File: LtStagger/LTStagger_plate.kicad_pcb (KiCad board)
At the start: 2 copper layers, 155 x 112 mm, 26 parts, among them K0 K00, K1 K01, K10 K10, K11 K11, K12 K12, K2 K02, K20 K20, K21 K21, K22 K22, K30 K30, K31 K31, K32 K32, K33 K33, K40 K40, K41 K41, K42 K42, K43 K43, K50 K50, K51 K51, K53 K53, SW1 Rotary_Encoder_Switch

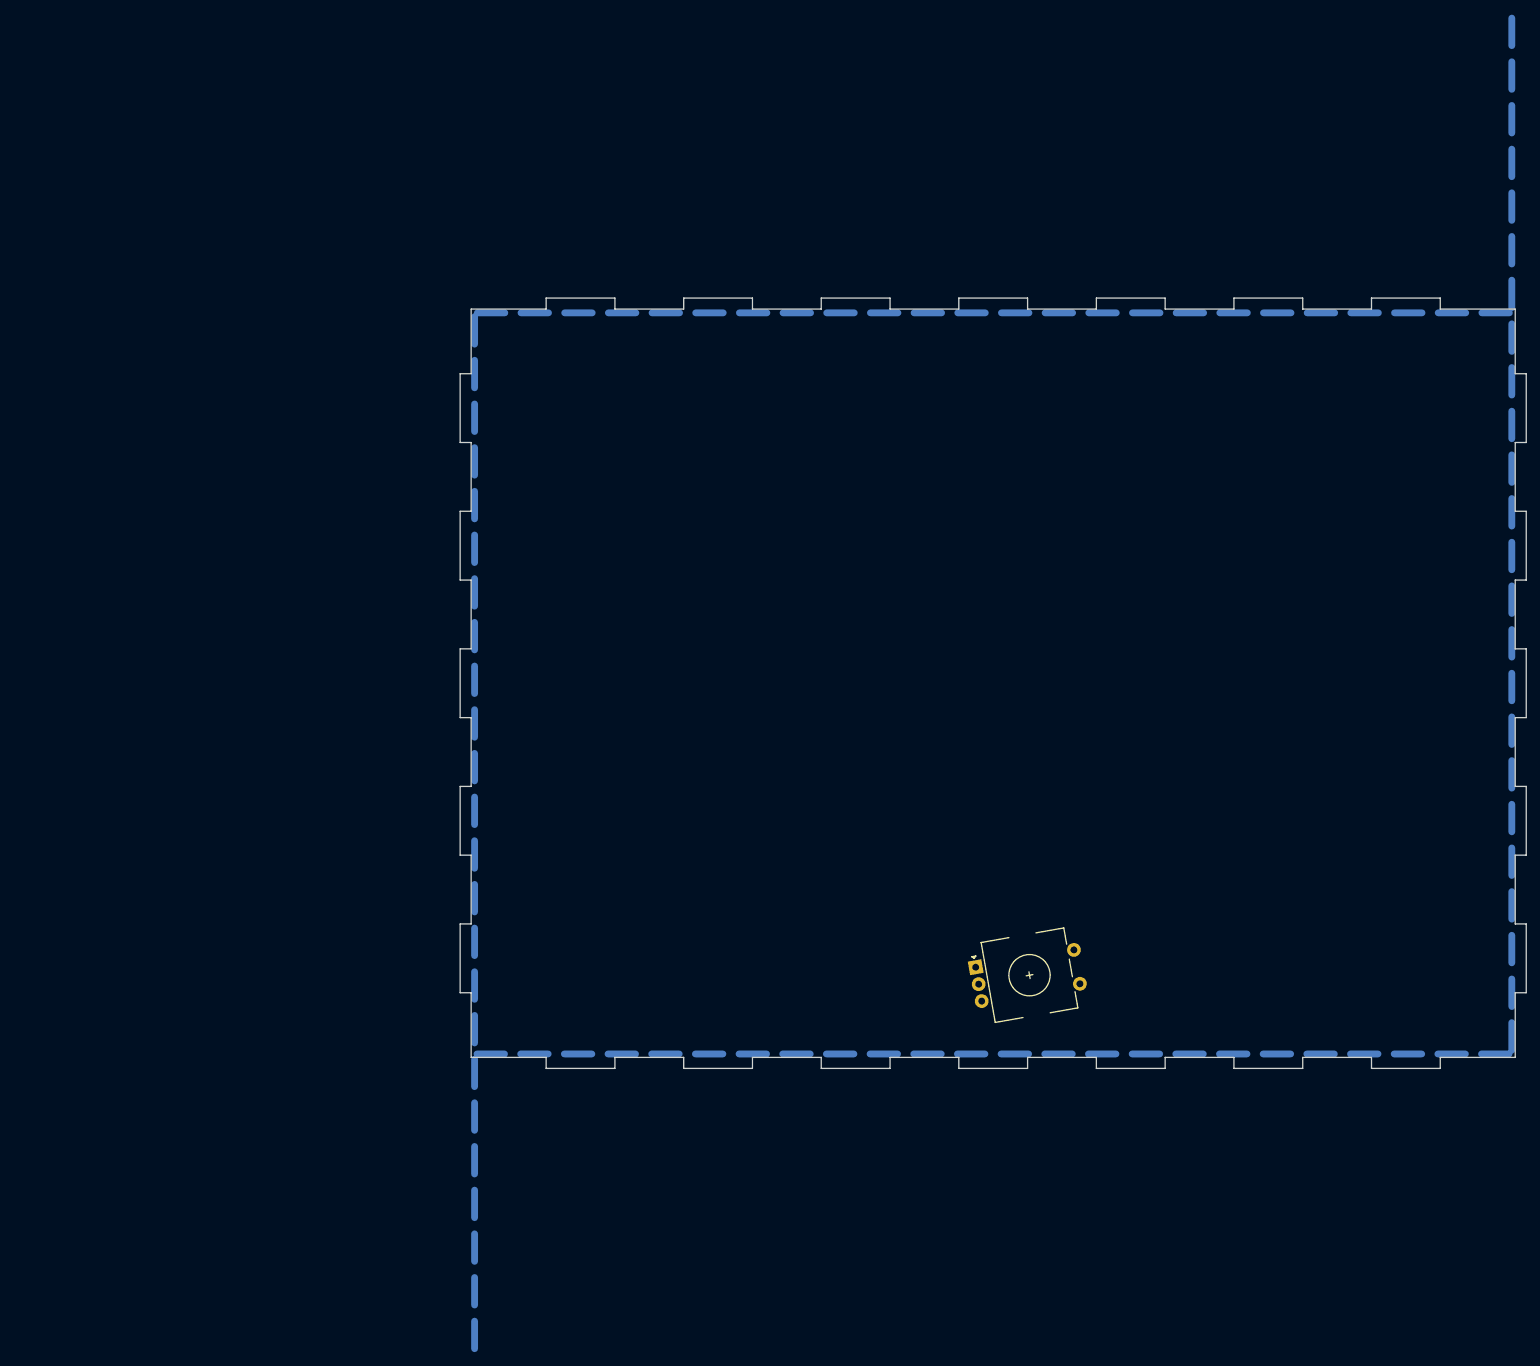
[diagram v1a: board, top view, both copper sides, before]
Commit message: Maybe ready for production
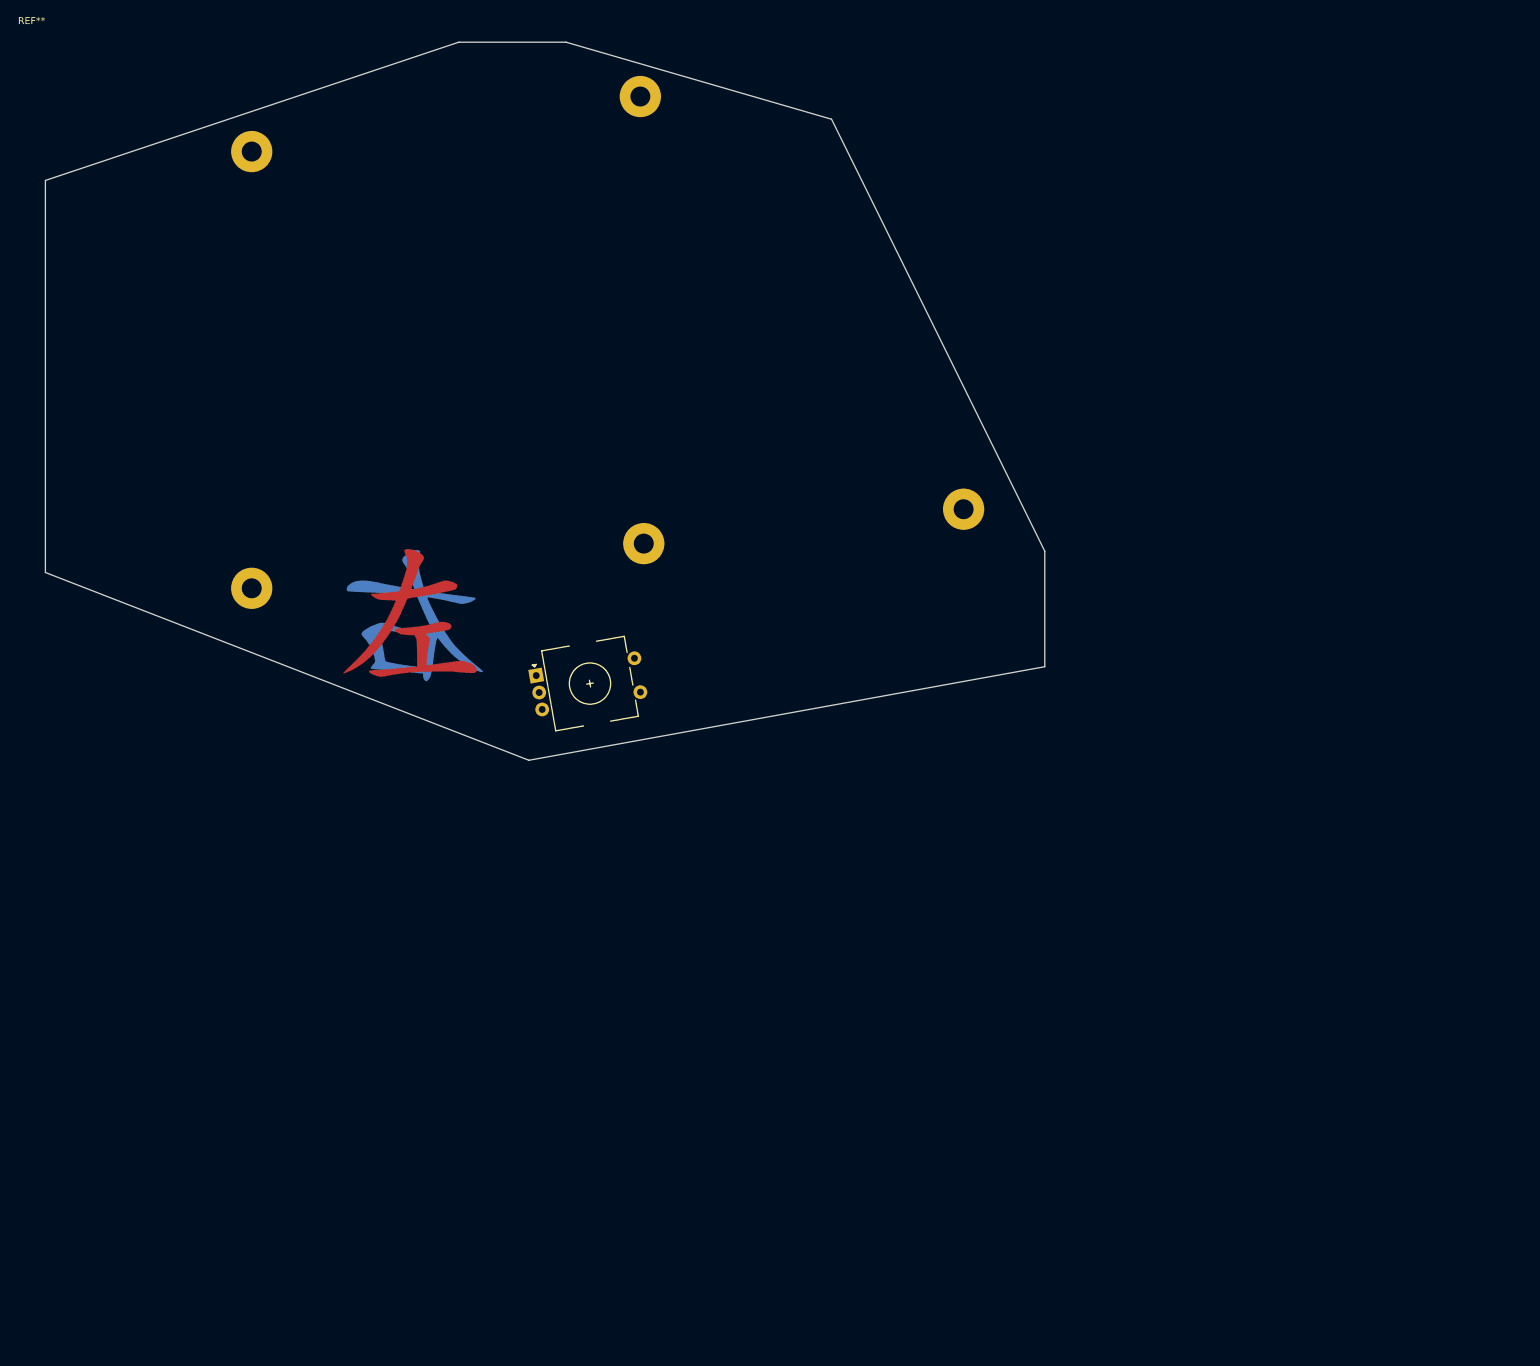
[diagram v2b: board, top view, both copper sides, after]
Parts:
- removed the REF** at (64.4, 45.5)
- removed the REF** at (215.2, 148.2)
- removed the REF** at (66.8, 150.7)
- removed the REF** at (66.8, 43.0)
- added ?: , Digi:Right, B.Cu at (55.3, 86.9)
- added ?: , Digi:Left, F.Cu at (55.8, 87.1)
- added REF**: Mounting Holes, Digi:Mounting Holes, F.Cu at (0.00, 0.00)
- moved K0 76.7 mm to (12.8, 32.2)
- moved K1 76.7 mm to (12.8, 51.2)
- moved K10 76.7 mm to (31.8, 32.2)
- moved K11 76.7 mm to (31.8, 51.2)
- moved K12 76.7 mm to (31.8, 70.3)
- moved K2 76.7 mm to (12.8, 70.3)
- moved K20 76.7 mm to (50.9, 19.6)
- moved K30 76.7 mm to (69.9, 12.9)
- moved K31 76.7 mm to (69.9, 32.0)
- moved K32 76.7 mm to (69.9, 51.0)
- moved K33 76.7 mm to (99.9, 93.5)
- moved K40 76.7 mm to (89.0, 23.1)
- moved K41 76.7 mm to (89.0, 42.2)
- moved K50 76.7 mm to (108.0, 23.1)
- moved K51 76.7 mm to (108.0, 42.2)
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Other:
- board size 155 x 112 mm -> 145.3 x 104.4 mm
